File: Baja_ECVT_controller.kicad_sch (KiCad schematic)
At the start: 37 parts, among them J1 Conn_01x04_Pin, J3 USB_C_Receptacle_USB2.0, J4 Micro_SD_Card_Det2, SW1 SW_Push, SW2 SW_SPDT, U1 STM32H725VGT6, U7 SN65HVD230, Y1 TSX-3225_16.0000MF09Z-AC6

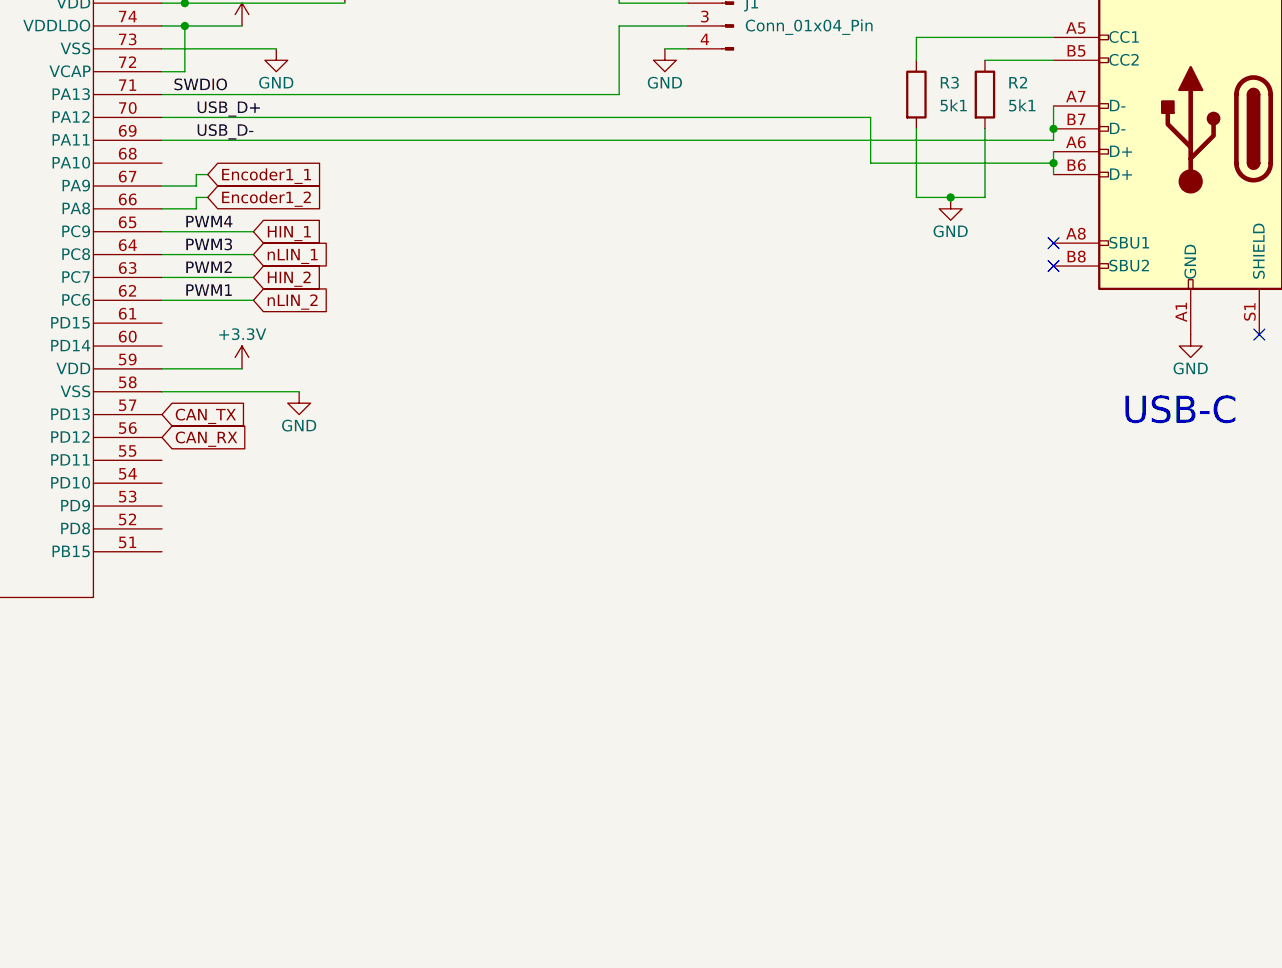
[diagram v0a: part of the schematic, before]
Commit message: Add files via upload
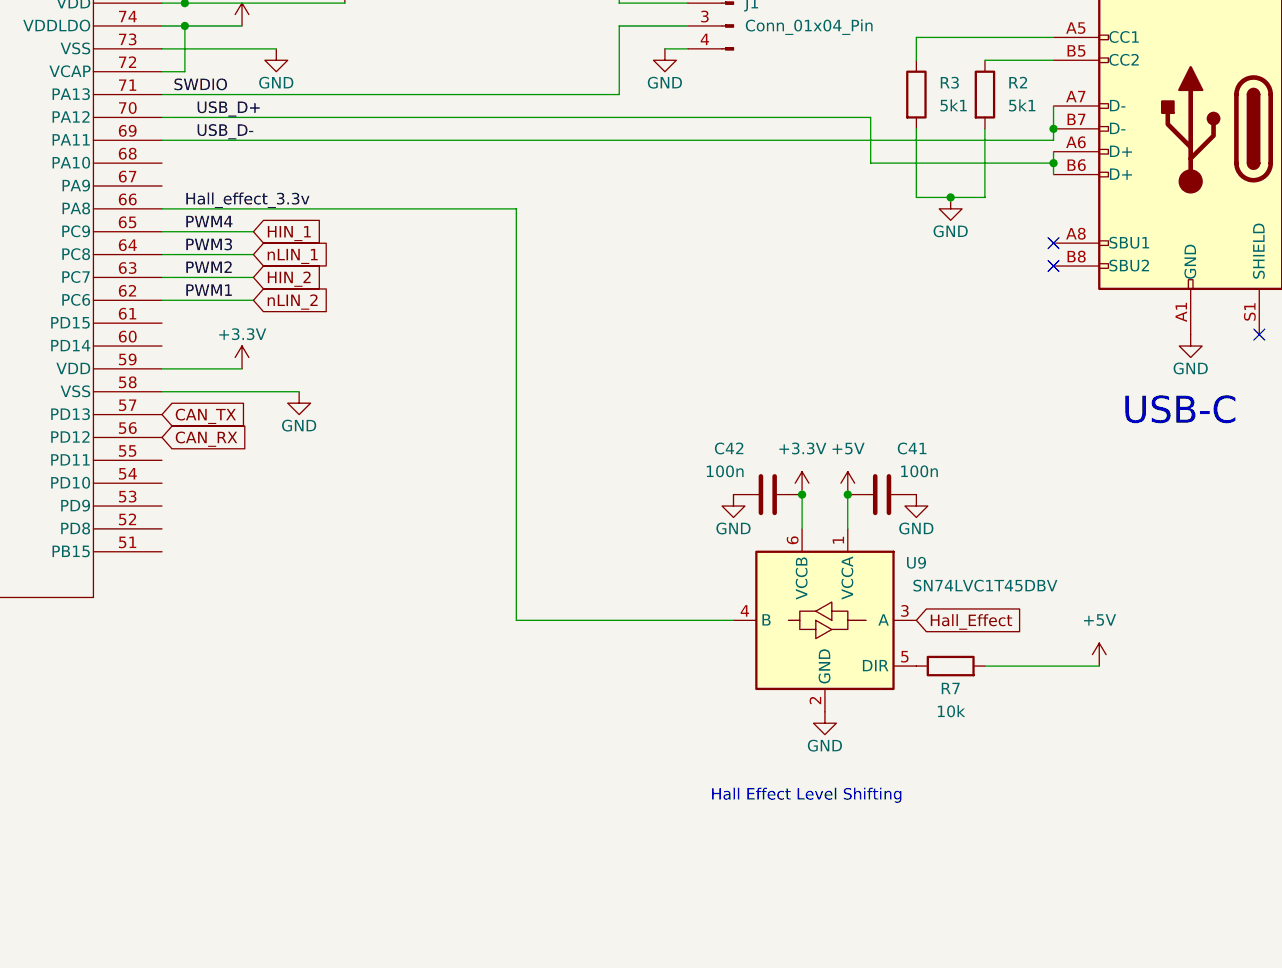
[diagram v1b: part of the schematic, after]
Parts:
- added C41, C42: 100n, symbol Device:C
- added R7: 10k, symbol Device:R
- added U9: SN74LVC1T45DBV, Package_TO_SOT_SMD:SOT-23-6, symbol Logic_LevelTranslator:SN74LVC1T45DBV
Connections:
- net +3.3V: now also C42.2, U9.6 (VCCB)
- net GND: now also C41.2, C42.1, U9.2 (GND)
- net Encoder1_1: no longer names the net of U1.67 (PA9)
- net Encoder1_2 renamed Hall_effect_3.3v
- net Hall_effect_3.3v: now also U9.4 (B)
- new net: R7.1, U9.5 (DIR)
- new net +5V: C41.1, R7.2, U9.1 (VCCA)
- new net Hall_Effect: U9.3 (A)
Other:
- note added: "Hall Effect Level Shifting"
